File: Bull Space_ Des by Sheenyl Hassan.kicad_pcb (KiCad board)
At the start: 2 copper layers, 45 x 77 mm, 37 parts, among them IC1 TEENSY_4.0, IC2 XB24CZ7PIT-004, J1 Screw_Terminal_01x06, Q1 AOI21357, Q2 2N7002, Q3 2N7002, Q4 2N7002, Q5 AOI21357, U1 VXO7803-1000, U2 Flight-Computer_Adafruit_GPS_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, U3 ADXL345, U4 BMP280, U6 Memory_Flash_W25Q32JVSS

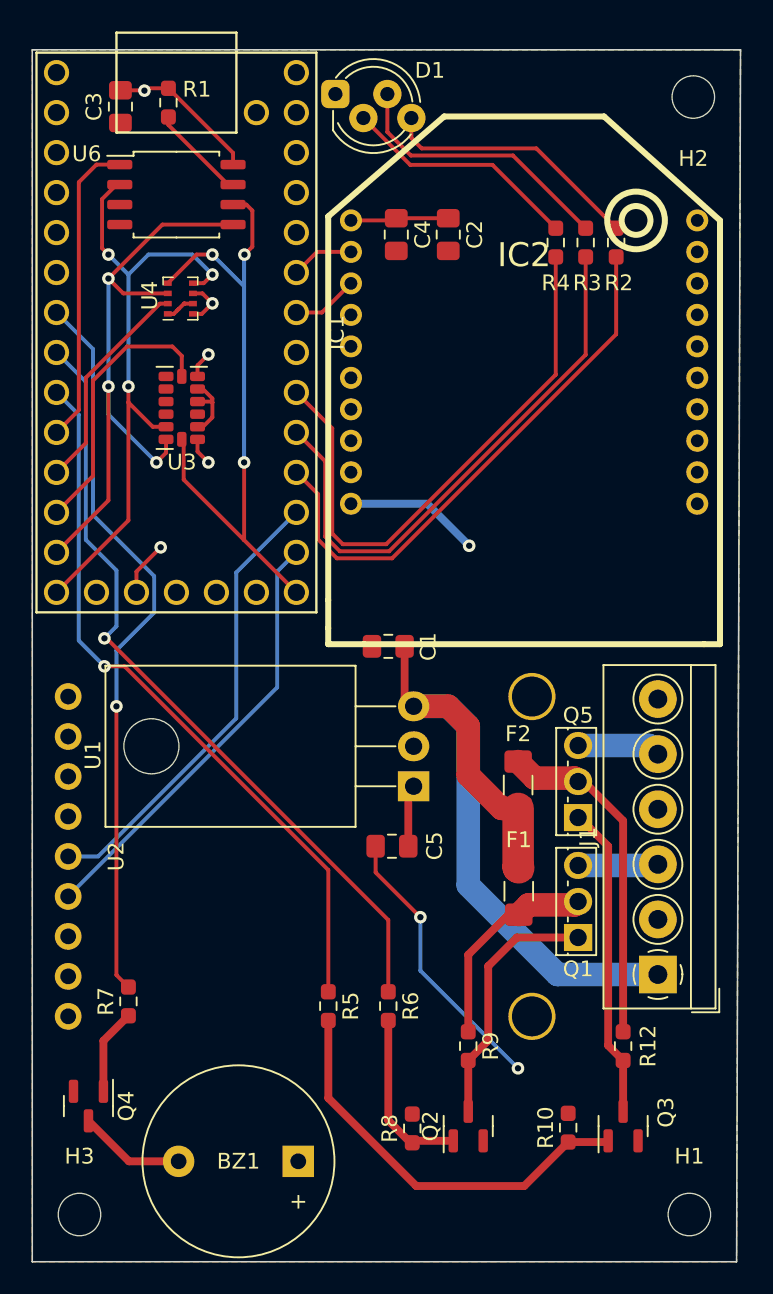
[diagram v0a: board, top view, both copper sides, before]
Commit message: Add files via upload
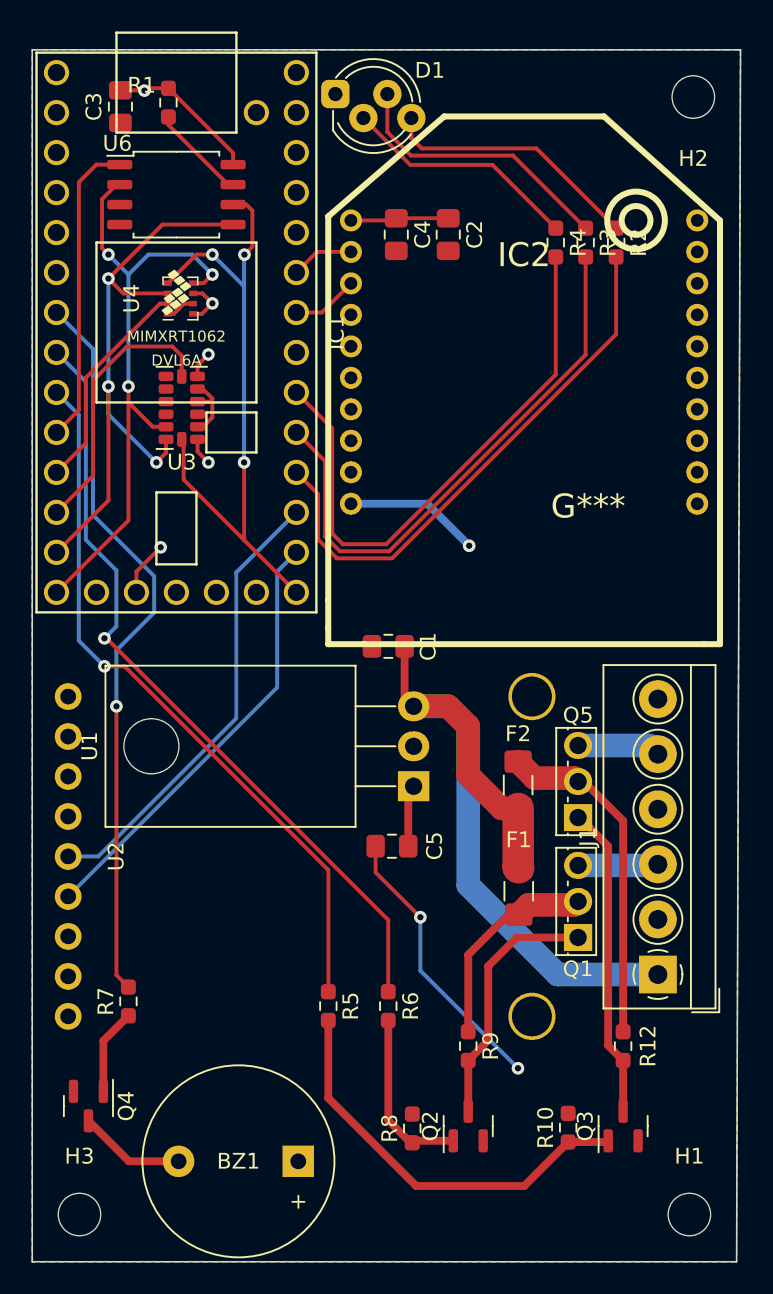
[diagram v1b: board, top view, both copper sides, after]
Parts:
- removed G1: UB-SEDS-Logo, Flight Computer:SEDS_logo_soldermask
- added G***: LOGO, misc diy:Seds logo v2, F.Cu at (107.3, 95.5)

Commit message: Revert "Add files via upload"
This reverts commit a89c25e643e2f36197d76d802668cdfff43c7fec.
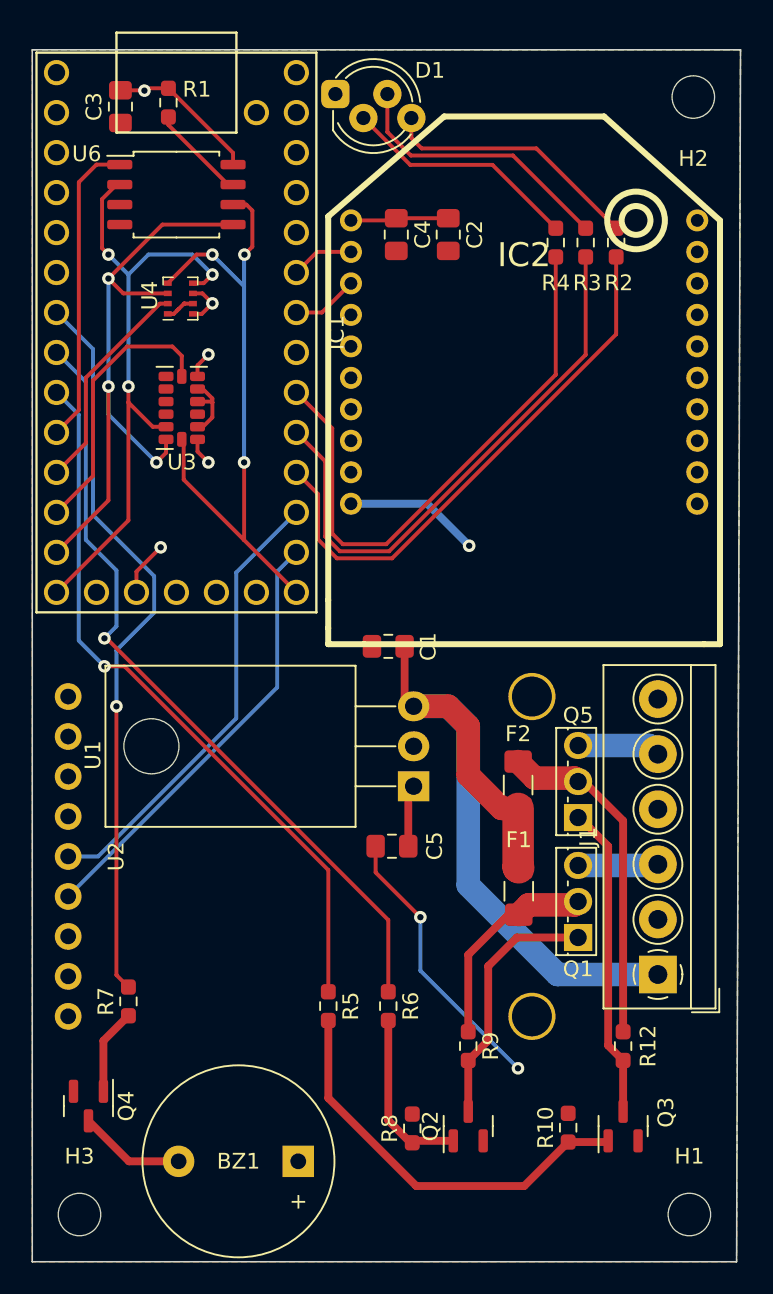
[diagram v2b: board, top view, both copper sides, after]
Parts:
- removed G***: LOGO, misc diy:Seds logo v2
- added G1: UB-SEDS-Logo, Flight Computer:SEDS_logo_soldermask, F.Cu at (101.3, 138.6)
